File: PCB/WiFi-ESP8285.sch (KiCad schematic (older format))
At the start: 20 parts, among them SW2 B3U-1000P, T1 1909763-1, U4 ESP8285, X3 FA-128_26.0000MF10Z-AC3

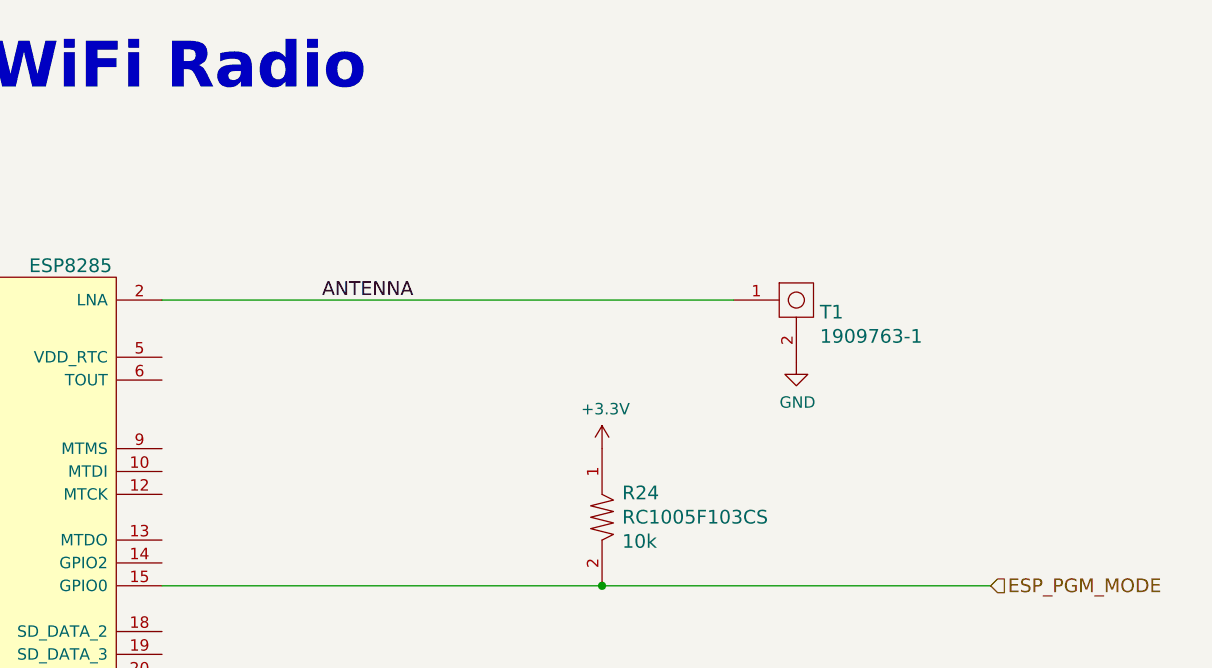
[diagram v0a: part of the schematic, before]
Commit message: Board Finished
Board finished
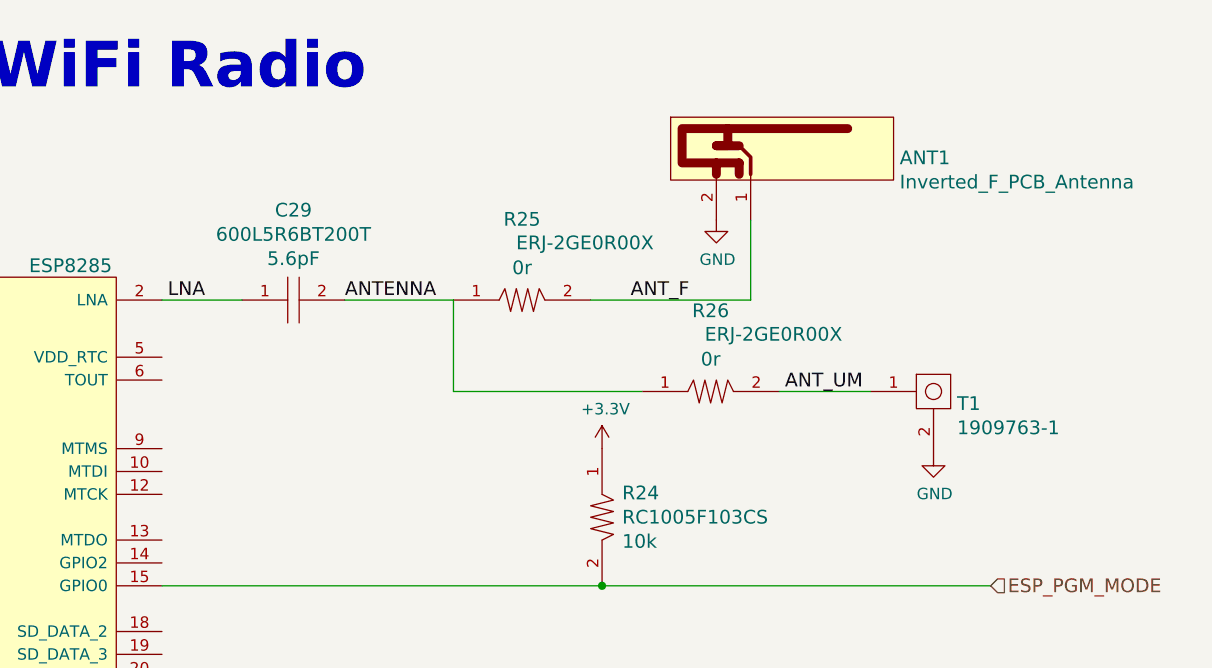
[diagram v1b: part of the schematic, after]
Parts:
- added ANT1: Inverted_F_PCB_Antenna, PCB_Footprints:PCB_IF_ANT_2.4G, symbol Inverted_F_PCB_Antenna
- added C29: 600L5R6BT200T, PCB_Footprints:C0402, symbol 600L5R6BT200T
- added R25, R26: ERJ-2GE0R00X, PCB_Footprints:R0402, symbol ERJ-2GE0R00X
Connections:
- net ANTENNA: now also C29.2, R25.1, R26.1; no longer T1.1, U4.2 (LNA)
- net GND: now also ANT1.2
- new net ANT_F: ANT1.1, R25.2
- new net ANT_UM: R26.2, T1.1
- new net LNA: C29.1, U4.2 (LNA)
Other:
- moved on the sheet: T1
